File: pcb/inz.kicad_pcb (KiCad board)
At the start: 4 copper layers, 410 parts, among them U1 AMS1117-3.3, U2 ESP32-S3-WROOM-1

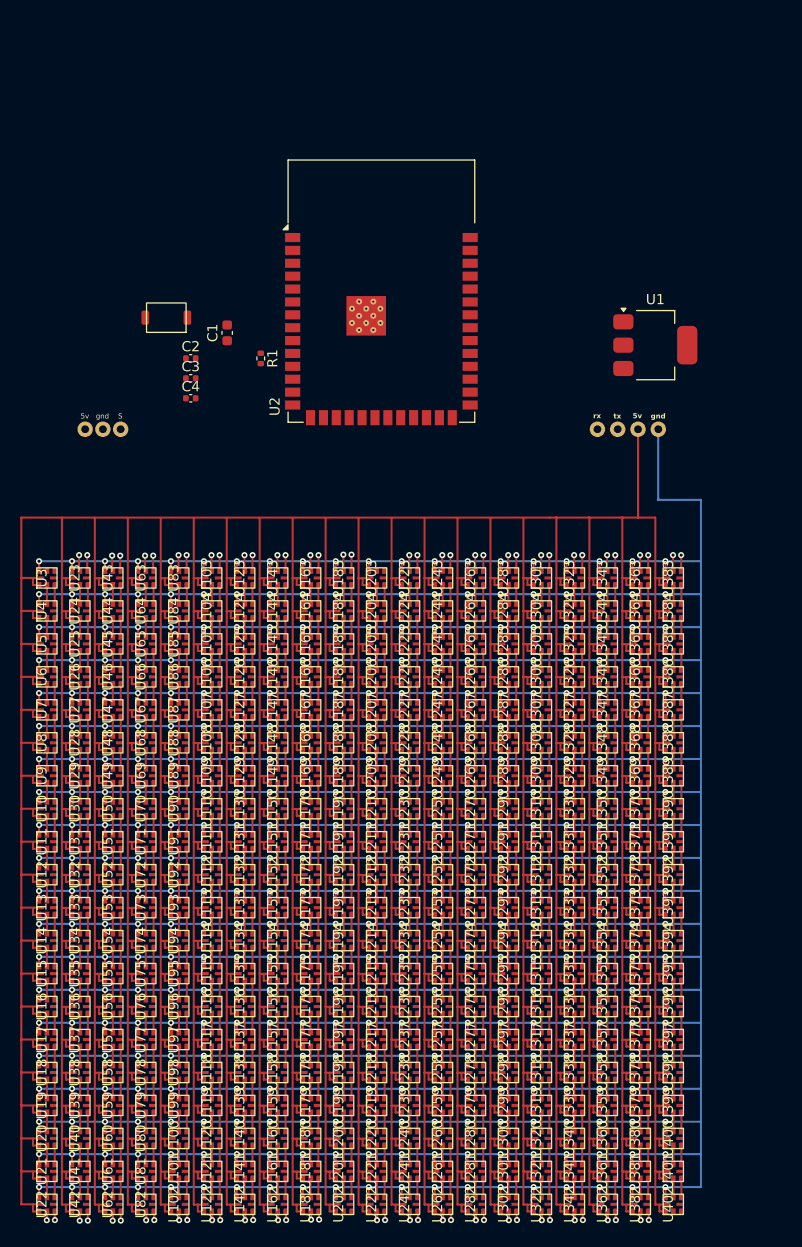
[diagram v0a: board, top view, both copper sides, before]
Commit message: +feat: finished second pcb design
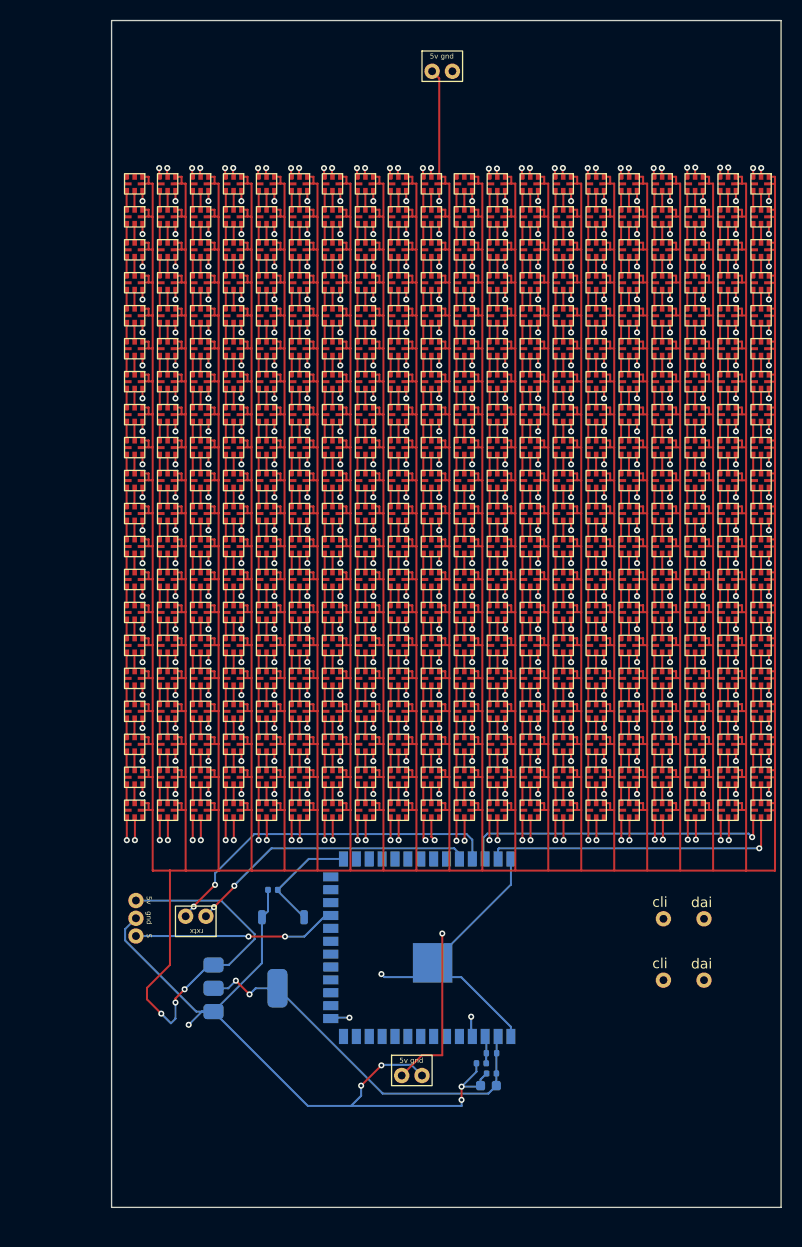
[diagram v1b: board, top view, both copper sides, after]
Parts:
- removed JT1: ~, LED_SMD:UART JT
- added LED_CON1: ~, RF_Module:led_con, F.Cu at (145.8, 132.6)
- added LED_CON2: ~, RF_Module:led_con, F.Cu at (145.8, 138.6)
- added pwr1: ~, RF_Module:5vgnd, F.Cu at (119.0, 148.0)
- added pwr2: ~, RF_Module:5vgnd, F.Cu at (122.0, 49.0)
- added rxtx1: ~, RF_Module:rxtx, F.Cu at (97.7, 132.3)
- C1, C2, C3, C4, R1, ST1, U1, U2: moved to B.Cu
- moved U22 122.8 mm to (153.4, 60.1), turned to -90 degrees
- moved U42 119.2 mm to (150.2, 60.1), turned to -90 degrees
- moved U21 117.5 mm to (153.4, 63.4), turned to -90 degrees
- moved U62 115.8 mm to (146.9, 60.1), turned to -90 degrees
- moved U402 113.8 mm to (91.7, 60.1), turned to -90 degrees
- moved U41 113.7 mm to (150.2, 63.4), turned to -90 degrees
- moved U82 112.7 mm to (143.7, 60.1), turned to -90 degrees
- moved U20 112.4 mm to (153.4, 66.6), turned to -90 degrees
- moved U382 110.9 mm to (94.9, 60.1), turned to -90 degrees
- moved U61 110.2 mm to (146.9, 63.4), turned to -90 degrees
- moved U102 110.0 mm to (140.4, 60.1), turned to -90 degrees
- moved U40 108.4 mm to (150.2, 66.6), turned to -90 degrees
- moved U362 108.3 mm to (98.2, 60.1), turned to -90 degrees
- moved U401 108.0 mm to (91.7, 63.4), turned to -90 degrees
- moved U122 107.5 mm to (137.2, 60.1), turned to -90 degrees
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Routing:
- net GND: track 1784.0 -> 1926.3 mm, vias 400 -> 386
- net +5V: track 2399.6 -> 2539.1 mm, vias 0 -> 4
- net Net-(LED_CON2-cli): track 0.00 -> 57.7 mm, vias 0 -> 2
- net Net-(LED_CON2-dai): track 0.00 -> 48.0 mm, vias 0 -> 2
- net Net-(LED_CON1-cli): track 0.00 -> 42.2 mm, vias 0 -> 1
- net Net-(LED_CON1-dai): track 0.00 -> 41.0 mm, vias 0 -> 1
- net Net-(U1-VO): track 0.00 -> 38.5 mm, vias 0 -> 2
- net UART_TX: track 0.00 -> 34.5 mm, vias 0 -> 2
- net UART_RX: track 0.00 -> 28.7 mm, vias 0 -> 2
- net Net-(JT2-S): track 0.00 -> 20.1 mm, vias 0 -> 2
- net Net-(U2-IO0): track 0.00 -> 11.5 mm
- net Net-(U2-EN): track 0.00 -> 2.70 mm
- net Net-(U382-CLO): track 70.0 -> 71.4 mm
- net Net-(U362-CLO): track 70.0 -> 71.4 mm
- net Net-(U342-CLO): track 70.0 -> 71.4 mm
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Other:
- board outline added: 66 x 117 mm
